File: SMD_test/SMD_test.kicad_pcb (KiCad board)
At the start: 4 copper layers, 46 x 49.4 mm, 7 parts, among them J1 Conn_01x03_Pin

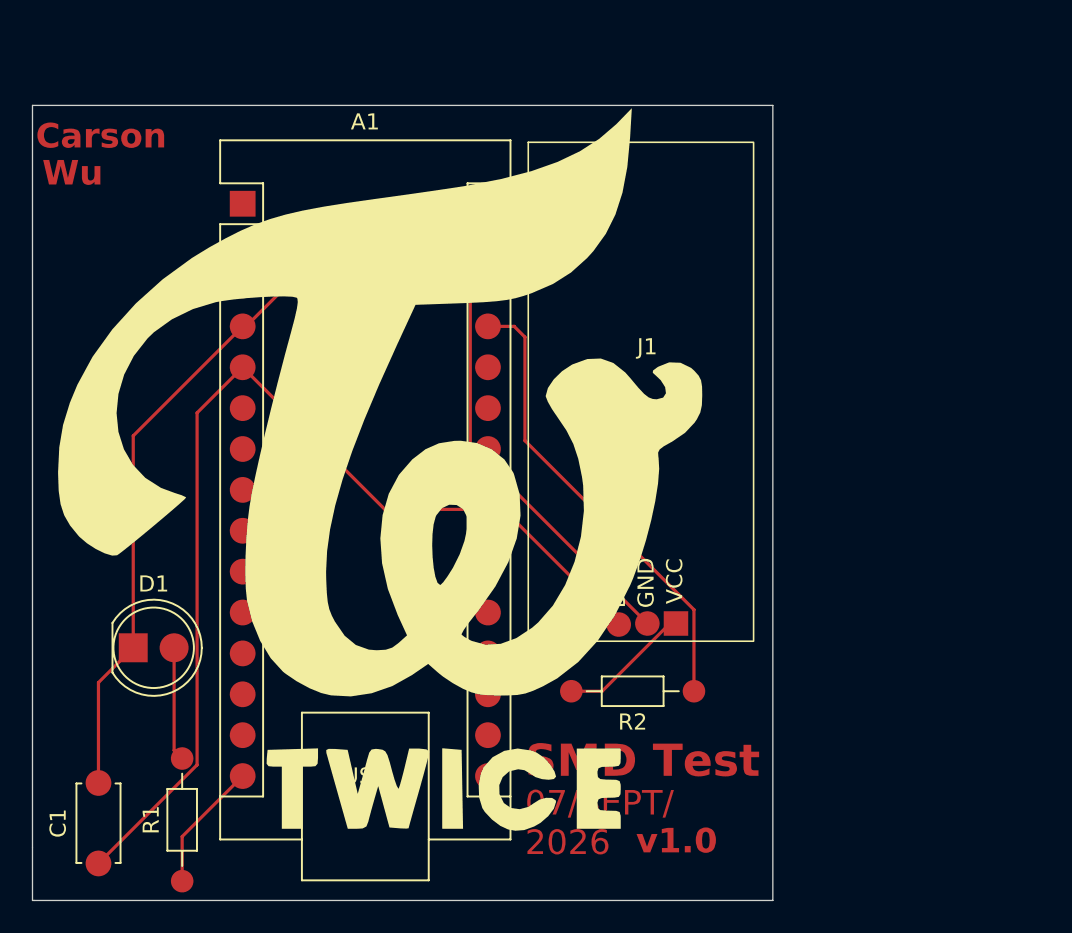
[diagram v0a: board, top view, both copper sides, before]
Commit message: updated SMD_test
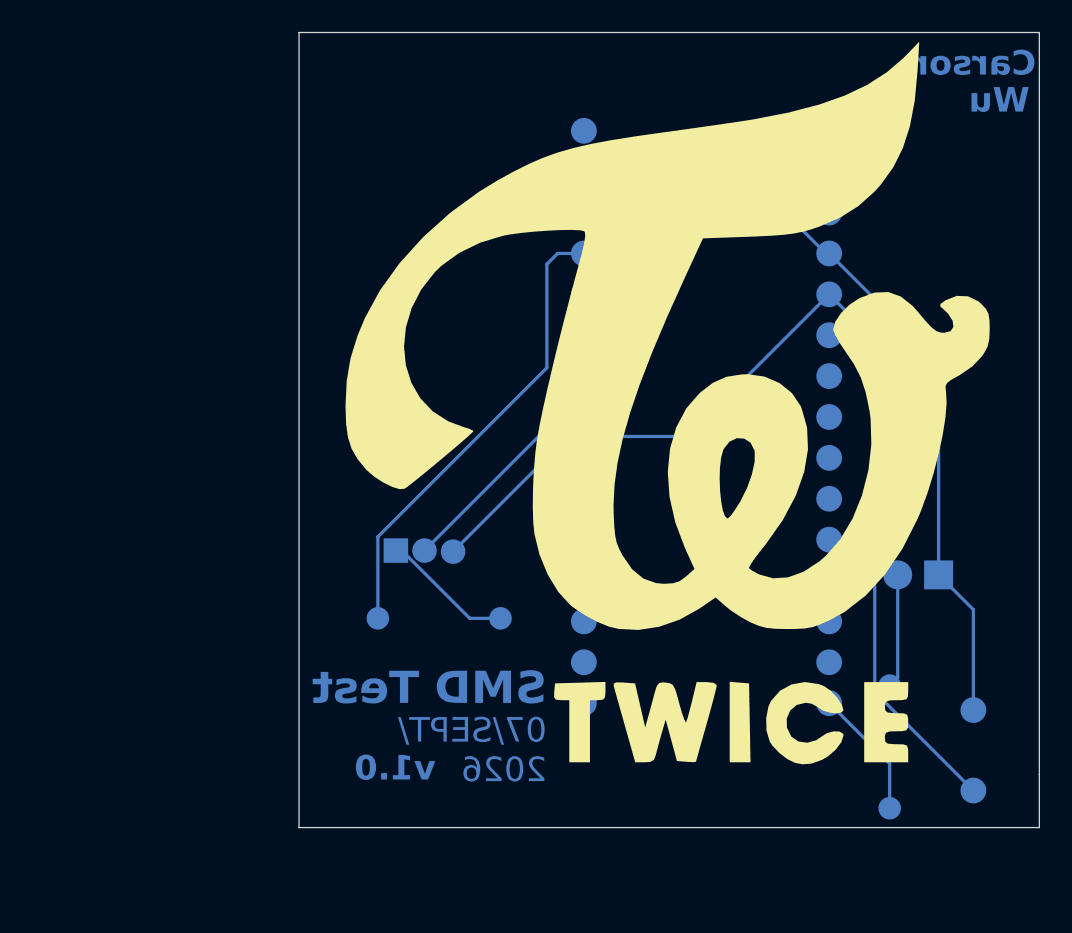
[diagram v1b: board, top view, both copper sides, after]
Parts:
- A1, C1, D1, J1, R1, R2: moved to B.Cu
- moved C1 54.5 mm to (163.6, 123.3)
- moved D1 50.2 mm to (161.4, 109.9), turned to 180 degrees
- moved R1 44.2 mm to (158.4, 124.4)
- moved A1 36.7 mm to (154.6, 82.3), turned to 180 degrees
- moved R2 20.2 mm to (126.6, 112.6), turned to 0 degrees
- moved G*** 18.3 mm to (144.6, 99.2)
- moved J1 14.6 mm to (129.5, 91.7), turned to 180 degrees
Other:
- outline, holes or cut-outs redrawn
